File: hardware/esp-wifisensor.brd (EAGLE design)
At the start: 57 x 54.5 mm, 16 parts

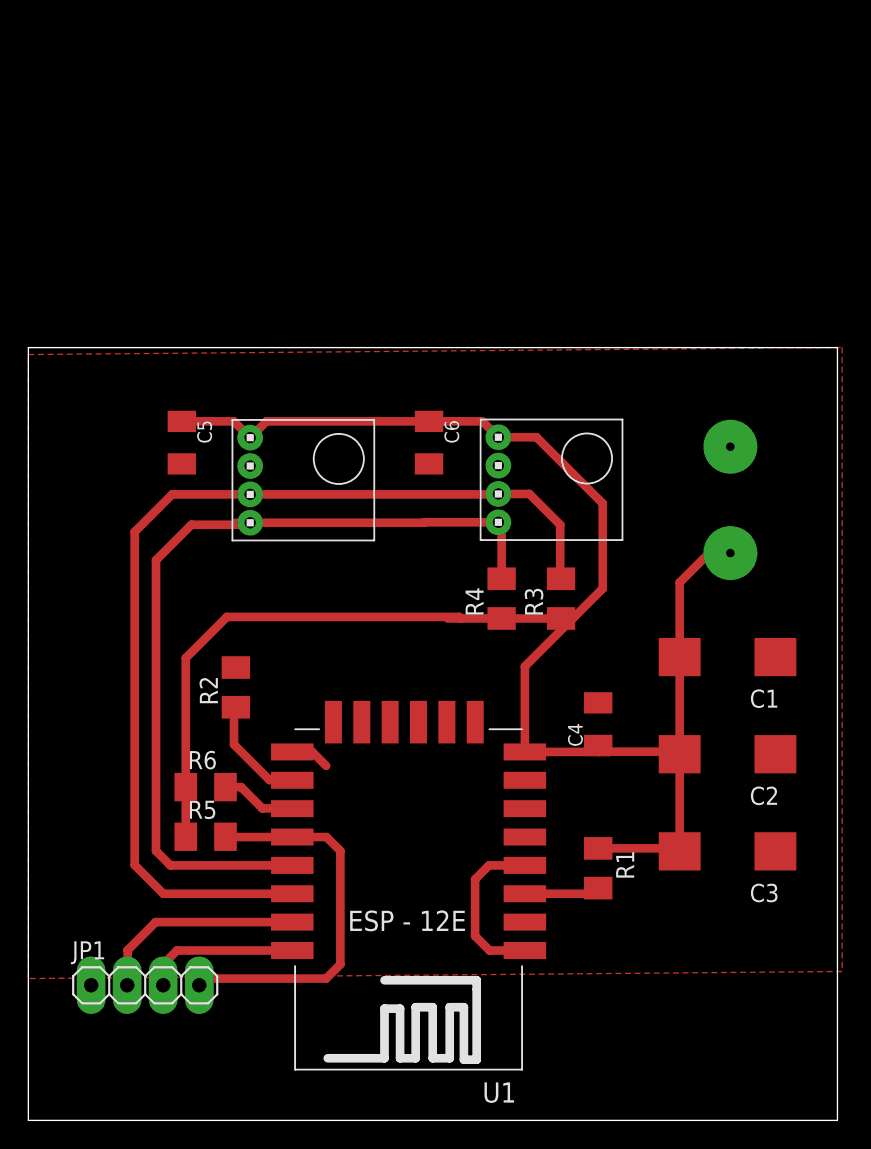
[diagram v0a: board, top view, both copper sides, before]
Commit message: hardware: updated schematics and pcb
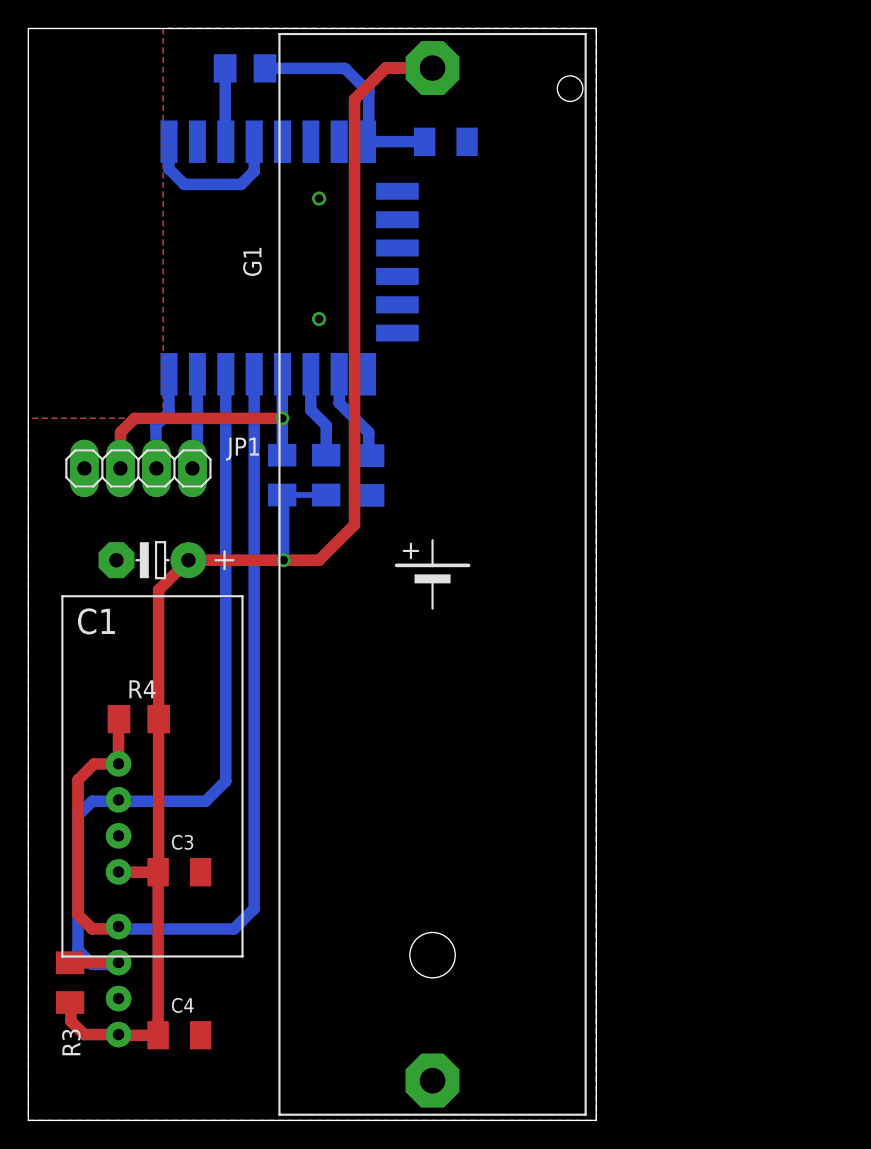
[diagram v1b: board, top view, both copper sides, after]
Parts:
- removed C5, C6: 100n, rcl:C1206K
- added G1: BHC-18650-1P, BHC-18650-1P:BHC-18650-1P
- C1: value 470u -> 1500u; device rcl:D/7343-31W -> ED1E152MNN1225:E5-13
- C2, C3: value 470u -> 100n; device rcl:D/7343-31W -> rcl:C1206K
- moved R1 61.7 mm to (15.3, 74.2), flipped to the bottom, turned to 0 degrees
- moved C2 47.5 mm to (29.4, 69.0), flipped to the bottom
- moved U1 44.3 mm to (15.7, 60.7), flipped to the bottom, turned to 270 degrees
- moved R3 44.0 mm to (2.94, 9.71)
- moved C1 41.1 mm to (8.75, 39.5)
- moved C3 38.7 mm to (10.7, 17.5), turned to 0 degrees
- moved C4 36.8 mm to (10.7, 6.00), turned to 0 degrees
- moved U$2 36.5 mm to (6.36, 9.86), flipped to the bottom, turned to 90 degrees
- moved JP1 36.4 mm to (7.76, 46.0), turned to 180 degrees
- moved U$1 35.9 mm to (6.36, 21.3), flipped to the bottom, turned to 90 degrees
- moved R4 27.0 mm to (7.79, 28.3), turned to 180 degrees
- moved R5 26.1 mm to (17.9, 45.5), flipped to the bottom, turned to 90 degrees
- moved R6 23.6 mm to (21.0, 45.5), flipped to the bottom, turned to 90 degrees
- moved R2 17.7 mm to (24.1, 45.5), flipped to the bottom, turned to 270 degrees
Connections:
- net GND: now also C2.2, C3.2, G1.-, JP1.4; no longer C2.-, C3.-, C5.2, C6.2, JP1.1
- net N$10: now also JP1.1; no longer JP1.2
- net N$5: now also JP1.3; no longer JP1.4
- net N$8: now also JP1.2; no longer JP1.3
- net VCC: now also C2.1, C3.1, G1.+; no longer C2.+, C3.+, C5.1, C6.1
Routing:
- net N$2: track 71.3 -> 56.5 mm
- net VCC: track 137.0 -> 123.2 mm
- net N$10: track 14.9 -> 7.30 mm
- net N$3: track 60.2 -> 67.3 mm
- net N$5: track 27.1 -> 20.2 mm, vias 0 -> 1
- net N$8: track 11.0 -> 7.03 mm
- net GND: track 3.41 -> 0.00 mm, vias 1 -> 2
- net N$6: track 6.49 -> 5.19 mm
- net N$4: track 7.84 -> 6.64 mm
- net N$1: track 11.8 -> 10.8 mm
- net N$7: track 5.34 -> 6.16 mm
- added copper zone on layer 16, net GND
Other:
- board size 57 x 54.5 mm -> 40 x 77 mm
